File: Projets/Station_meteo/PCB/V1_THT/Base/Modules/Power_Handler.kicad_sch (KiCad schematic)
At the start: 4 parts, among them Q7 FDS4559, Q8 2N7000

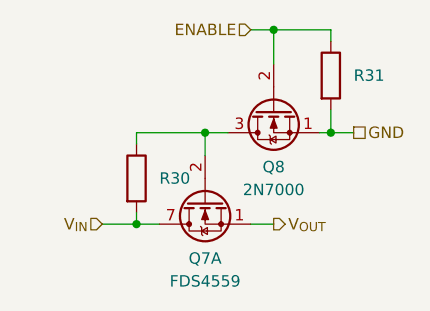
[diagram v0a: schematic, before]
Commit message: Update
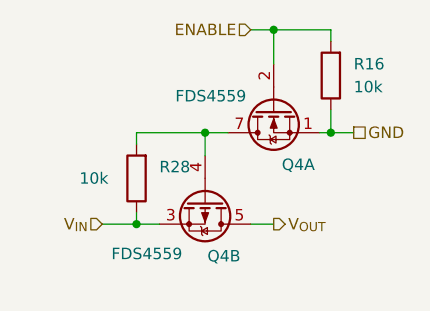
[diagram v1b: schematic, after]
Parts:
- removed Q7: FDS4559, Package_SO:SOIC-8_3.9x4.9mm_P1.27mm, symbol Transistor_FET:FDS4559
- removed Q8: 2N7000, Package_TO_SOT_THT:TO-92_Inline, symbol Transistor_FET:2N7000
- removed R30, R31: 10k, Resistor_THT:R_Axial_DIN0207_L6.3mm_D2.5mm_P7.62mm_Horizontal, symbol CREPP_Resistors:Resistor_THT_250mW (standard)
- added Q4: FDS4559, Package_SO:SOIC-8_3.9x4.9mm_P1.27mm, symbol Transistor_FET:FDS4559
- added R16, R28: 10k, Resistor_THT:R_Axial_DIN0207_L6.3mm_D2.5mm_P7.62mm_Horizontal, symbol Device:R
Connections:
- net ENABLE: now also Q4.2 (G), R16.2
- net GND: now also Q4.1 (S), R16.1
- net V_{IN}: now also Q4.3 (1), R28.1
- net V_{OUT}: now also Q4.5 (D), Q4.6 (D)
- new net: Q4.4 (G), Q4.7 (D), Q4.8 (D), R28.2
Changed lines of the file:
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@@
 	)
 	(symbol
-		(lib_id "CREPP_Resistors:Resistor_THT_250mW (standard)")
-		(at 109.22 54.61 0)
+		(lib_id "Device:R")
+		(at 109.22 54.61 180)
 		(unit 1)
 		(exclude_from_sim no)
@@
 		(dnp no)
 		(fields_autoplaced yes)
-		(property "Reference" "R31"
-			(at 111.76 54.6099 0)
-			(effects
-				(font
-					(size 1.27 1.27)
-				)
-				(justify left)
+		(property "Reference" "R16"
+			(at 111.76 53.3399 0)
+			(effects
+				(font
+					(size 1.27 1.27)
+				)
+				(justify right)
 			)
 		)
 		(property "Value" "10k"
-			(at 119.126 52.07 0)
-			(effects
-				(font
-					(size 1.27 1.27)
-				)
-				(hide yes)
+			(at 111.76 55.8799 0)
+			(effects
+				(font
+					(size 1.27 1.27)
+				)
+				(justify right)
 			)
 		)
 		(property "Footprint" "Resistor_THT:R_Axial_DIN0207_L6.3mm_D2.5mm_P7.62mm_Horizontal"
-			(at 107.442 54.61 90)
+			(at 110.998 54.61 90)
 			(effects
 				(font
@@
 			)
 		)
-		(property "Description" "Standard resistor - 1/4W - THT version"
+		(property "Description" ""
 			(at 109.22 54.61 0)
 			(effects
@@
 			)
 		)
+		(pin "1"
+		)
 		(pin "2"
-		)
-		(pin "1"
 		)
 		(instances
 			(project "Base"
 				(path "/4bc9f80e-0a24-4618-ba5d-3a118070c43e/16c1cf0a-7f1e-4c3f-ad57-311ae10c4222"
-					(reference "R31")
+					(reference "R16")
 					(unit 1)
 				)
 				(path "/4bc9f80e-0a24-4618-ba5d-3a118070c43e/6abfbb7c-4a96-4b3c-bae8-1f7b8b6c7442"
-					(reference "R17")
+					(reference "R15")
 					(unit 1)
 				)
 				(path "/4bc9f80e-0a24-4618-ba5d-3a118070c43e/a5c65fee-c30f-43d3-8fce-13d00ed1041d"
-					(reference "R32")
+					(reference "R1")
 					(unit 1)
 				)
 				(path "/4bc9f80e-0a24-4618-ba5d-3a118070c43e/a63dc76b-6380-494c-9d24-5850142aff19"
-					(reference "R15")
-					(unit 1)
-				)
-				(path "/4bc9f80e-0a24-4618-ba5d-3a118070c43e/b189c293-6c32-4865-840c-f316708689bc"
-					(reference "R33")
+					(reference "R14")
 					(unit 1)
 				)
@@
 	(symbol
 		(lib_id "Transistor_FET:FDS4559")
-		(at 95.25 68.58 90)
-		(mirror x)
-		(unit 1)
+		(at 95.25 68.58 270)
+		(unit 2)
 		(exclude_from_sim no)
 		(in_bom yes)
 		(on_board yes)
 		(dnp no)
-		(fields_autoplaced yes)
-		(property "Reference" "Q7"
-			(at 95.25 74.93 90)
-			(effects
-				(font
-					(size 1.27 1.27)
-				)
+		(property "Reference" "Q4"
+			(at 95.504 74.676 90)
+			(effects
+				(font
+					(size 1.27 1.27)
+				)
+				(justify left)
 			)
 		)
 		(property "Value" "FDS4559"
-			(at 95.25 77.47 90)
-			(effects
-				(font
-					(size 1.27 1.27)
-				)
+			(at 84.836 74.422 90)
+			(effects
+				(font
+					(size 1.27 1.27)
+				)
+				(justify left)
 			)
 		)
 		(property "Footprint" "Package_SO:SOIC-8_3.9x4.9mm_P1.27mm"
-			(at 97.155 73.66 0)
+			(at 93.345 73.66 0)
 			(effects
 				(font
@@
 		)
 		(property "Datasheet" "https://www.onsemi.com/pub/Collateral/FDS4559-D.PDF"
-			(at 99.06 73.66 0)
+			(at 91.44 73.66 0)
 			(effects
 				(font
@@
 			)
 		)
+		(pin "1"
+		)
+		(pin "3"
+		)
+		(pin "6"
+		)
+		(pin "2"
+		)
+		(pin "8"
+		)
+		(pin "7"
+		)
 		(pin "4"
 		)
-		(pin "6"
-		)
-		(pin "1"
-		)
 		(pin "5"
-		)
-		(pin "3"
-		)
-		(pin "8"
-		)
-		(pin "7"
-		)
-		(pin "2"
 		)
 		(instances
 			(project "Base"
 				(path "/4bc9f80e-0a24-4618-ba5d-3a118070c43e/16c1cf0a-7f1e-4c3f-ad57-311ae10c4222"
-					(reference "Q7")
-					(unit 1)
+					(reference "Q4")
+					(unit 2)
 				)
 				(path "/4bc9f80e-0a24-4618-ba5d-3a118070c43e/6abfbb7c-4a96-4b3c-bae8-1f7b8b6c7442"
-					(reference "Q5")
-					(unit 1)
+					(reference "Q3")
+					(unit 2)
 				)
 				(path "/4bc9f80e-0a24-4618-ba5d-3a118070c43e/a5c65fee-c30f-43d3-8fce-13d00ed1041d"
 					(reference "Q1")
-					(unit 1)
+					(unit 2)
 				)
 				(path "/4bc9f80e-0a24-4618-ba5d-3a118070c43e/a63dc76b-6380-494c-9d24-5850142aff19"
 					(reference "Q2")
-					(unit 1)
-				)
-				(path "/4bc9f80e-0a24-4618-ba5d-3a118070c43e/b189c293-6c32-4865-840c-f316708689bc"
-					(reference "Q3")
-					(unit 1)
+					(unit 2)
 				)
 			)
@@
 	)
 	(symbol
-		(lib_id "Transistor_FET:2N7000")
+		(lib_id "Transistor_FET:FDS4559")
 		(at 102.87 58.42 90)
 		(mirror x)
@@
 		(on_board yes)
 		(dnp no)
-		(fields_autoplaced yes)
-		(property "Reference" "Q8"
-			(at 102.87 64.77 90)
-			(effects
-				(font
-					(size 1.27 1.27)
-				)
-			)
-		)
-		(property "Value" "2N7000"
-			(at 102.87 67.31 90)
-			(effects
-				(font
-					(size 1.27 1.27)
-				)
-			)
-		)
-		(property "Footprint" "Package_TO_SOT_THT:TO-92_Inline"
+		(property "Reference" "Q4"
+			(at 107.442 64.516 90)
+			(effects
+				(font
+					(size 1.27 1.27)
+				)
+				(justify left)
+			)
+		)
+		(property "Value" "FDS4559"
+			(at 99.822 56.896 90)
+			(effects
+				(font
+					(size 1.27 1.27)
+				)
+				(justify left)
+			)
+		)
+		(property "Footprint" "Package_SO:SOIC-8_3.9x4.9mm_P1.27mm"
 			(at 104.775 63.5 0)
 			(effects
@@
 			)
 		)
-		(property "Datasheet" "https://www.vishay.com/docs/70226/70226.pdf"
+		(property "Datasheet" "https://www.onsemi.com/pub/Collateral/FDS4559-D.PDF"
 			(at 106.68 63.5 0)
 			(effects
@@
 			)
 		)
-		(property "Description" "0.2A Id, 200V Vds, N-Channel MOSFET, 2.6V Logic Level, TO-92"
+		(property "Description" "4.5A Id, 60V Vds, Dual N and P Channel MOSFET, 55mOhm Ron, 10V Vgs, SO8L"
 			(at 102.87 58.42 0)
 			(effects
@@
 			)
 		)
+		(pin "1"
+		)
 		(pin "3"
 		)
+		(pin "6"
+		)
 		(pin "2"
 		)
-		(pin "1"
+		(pin "8"
+		)
+		(pin "7"
+		)
+		(pin "4"
+		)
+		(pin "5"
 		)
 		(instances
 			(project "Base"
 				(path "/4bc9f80e-0a24-4618-ba5d-3a118070c43e/16c1cf0a-7f1e-4c3f-ad57-311ae10c4222"
-					(reference "Q8")
+					(reference "Q4")
 					(unit 1)
 				)
 				(path "/4bc9f80e-0a24-4618-ba5d-3a118070c43e/6abfbb7c-4a96-4b3c-bae8-1f7b8b6c7442"
-					(reference "Q6")
+					(reference "Q3")
 					(unit 1)
 				)
 				(path "/4bc9f80e-0a24-4618-ba5d-3a118070c43e/a5c65fee-c30f-43d3-8fce-13d00ed1041d"
-					(reference "Q9")
+					(reference "Q1")
 					(unit 1)
 				)
 				(path "/4bc9f80e-0a24-4618-ba5d-3a118070c43e/a63dc76b-6380-494c-9d24-5850142aff19"
-					(reference "Q4")
-					(unit 1)
-				)
-				(path "/4bc9f80e-0a24-4618-ba5d-3a118070c43e/b189c293-6c32-4865-840c-f316708689bc"
-					(reference "Q10")
+					(reference "Q2")
 					(unit 1)
 				)
@@
 	)
 	(symbol
-		(lib_id "CREPP_Resistors:Resistor_THT_250mW (standard)")
-		(at 87.63 66.04 0)
+		(lib_id "Device:R")
+		(at 87.63 66.04 180)
 		(unit 1)
 		(exclude_from_sim no)
@@
 		(on_board yes)
 		(dnp no)
-		(fields_autoplaced yes)
-		(property "Reference" "R30"
-			(at 90.17 66.0399 0)
-			(effects
-				(font
-					(size 1.27 1.27)
-				)
-				(justify left)
+		(property "Reference" "R28"
+			(at 90.17 64.7699 0)
+			(effects
+				(font
+					(size 1.27 1.27)
+				)
+				(justify right)
 			)
 		)
 		(property "Value" "10k"
-			(at 97.536 63.5 0)
-			(effects
-				(font
-					(size 1.27 1.27)
-				)
-				(hide yes)
+			(at 81.28 66.04 0)
+			(effects
+				(font
+					(size 1.27 1.27)
+				)
+				(justify right)
 			)
 		)
 		(property "Footprint" "Resistor_THT:R_Axial_DIN0207_L6.3mm_D2.5mm_P7.62mm_Horizontal"
-			(at 85.852 66.04 90)
+			(at 89.408 66.04 90)
 			(effects
 				(font
@@
 			)
 		)
-		(property "Description" "Standard resistor - 1/4W - THT version"
+		(property "Description" ""
 			(at 87.63 66.04 0)
 			(effects
@@
 			)
 		)
+		(pin "1"
+		)
 		(pin "2"
-		)
-		(pin "1"
 		)
 		(instances
 			(project "Base"
 				(path "/4bc9f80e-0a24-4618-ba5d-3a118070c43e/16c1cf0a-7f1e-4c3f-ad57-311ae10c4222"
-					(reference "R30")
+					(reference "R28")
 					(unit 1)
 				)
 				(path "/4bc9f80e-0a24-4618-ba5d-3a118070c43e/6abfbb7c-4a96-4b3c-bae8-1f7b8b6c7442"
-					(reference "R16")
+					(reference "R19")
 					(unit 1)
 				)
 				(path "/4bc9f80e-0a24-4618-ba5d-3a118070c43e/a5c65fee-c30f-43d3-8fce-13d00ed1041d"
-					(reference "R1")
+					(reference "R2")
 					(unit 1)
 				)
 				(path "/4bc9f80e-0a24-4618-ba5d-3a118070c43e/a63dc76b-6380-494c-9d24-5850142aff19"
-					(reference "R14")
-					(unit 1)
-				)
-				(path "/4bc9f80e-0a24-4618-ba5d-3a118070c43e/b189c293-6c32-4865-840c-f316708689bc"
-					(reference "R2")
-					(unit 1)
-				)
+					(reference "R18")
+					(unit 1)
+				)
